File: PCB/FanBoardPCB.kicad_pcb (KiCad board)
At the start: 2 copper layers, 40 x 37.9 mm, 29 parts, among them J1 Conn_01x02_Pin, J2 Conn_01x02_Pin, J3 Conn_01x02_Pin, J4 Conn_01x02_Pin, J5 FanBrdConn, Q1 IRLML0030, Q2 IRLML0030, Q3 IRLML0030, Q4 IRLML0030

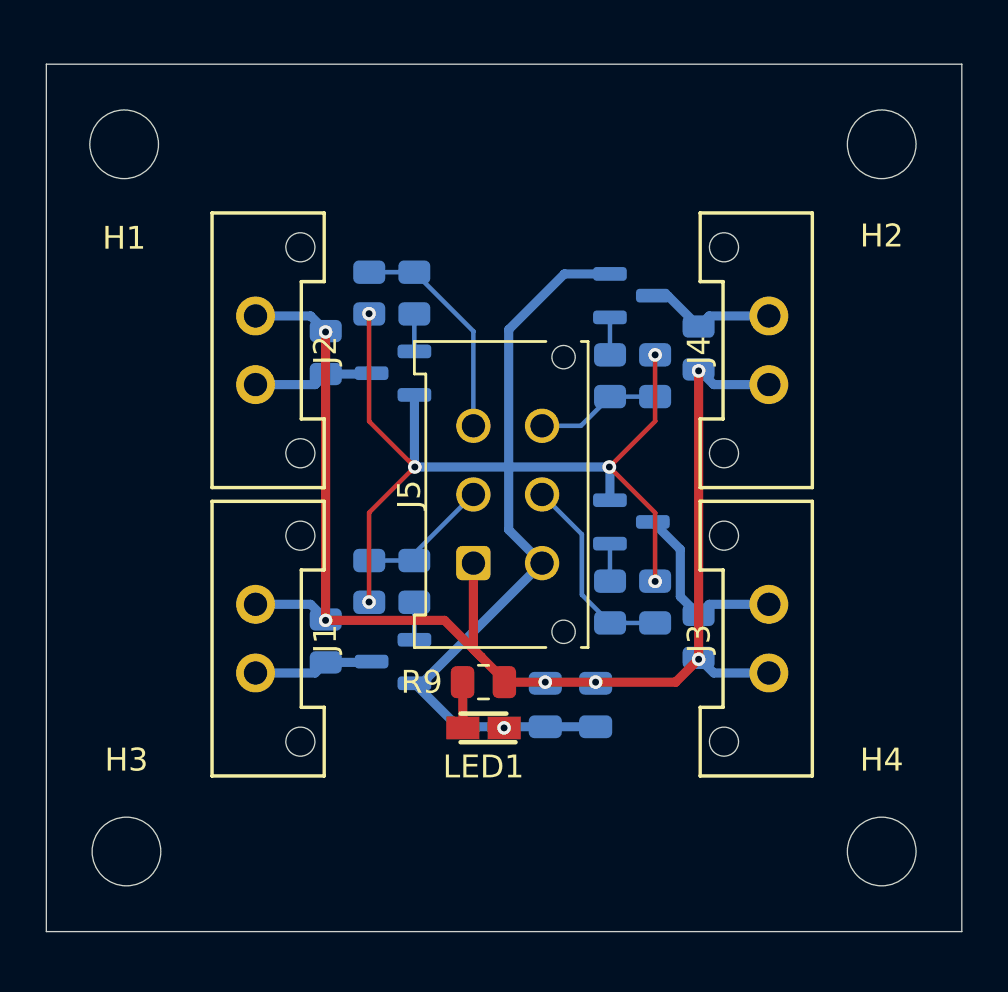
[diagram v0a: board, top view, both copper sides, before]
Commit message: fixed
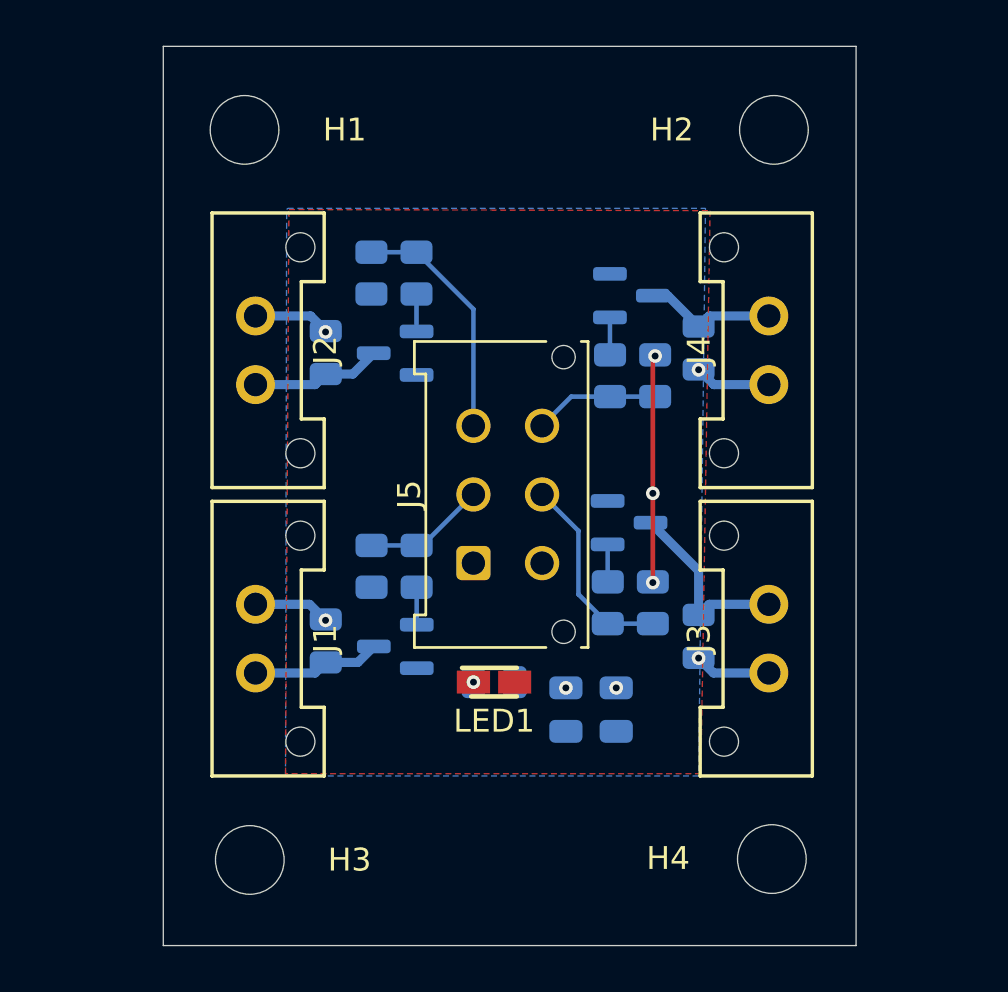
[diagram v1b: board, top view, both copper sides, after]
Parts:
- R9: moved to B.Cu
- moved H3 5.40 mm to (76.4, 130.6)
- moved H1 5.30 mm to (76.2, 98.7)
- moved H4 4.81 mm to (99.2, 130.5)
- moved H2 4.75 mm to (99.3, 98.7)
- moved LED1 2.05 mm to (87.1, 122.8), turned to 0 degrees
- moved C1 0.92 mm to (92.4, 124.0)
- moved C2 0.92 mm to (90.2, 124.0)
- moved Q2 0.88 mm to (82.7, 108.4)
- moved R3 0.88 mm to (81.7, 104.9)
- moved R4 0.88 mm to (83.7, 104.9)
- moved Q1 0.67 mm to (82.7, 121.2)
- moved R2 0.67 mm to (83.7, 117.7)
- moved R1 0.67 mm to (81.7, 117.7)
- moved R9 0.46 mm to (87.1, 122.8), turned to 0 degrees
- moved Q3 0.11 mm to (93.0, 115.8)
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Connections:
- LED1 pad 1: GNDPWR -> Net-(LED1-K)
- LED1 pad 2: Net-(LED1-A) -> +12V
- R9 pad 1: +12V -> Net-(LED1-K)
- R9 pad 2: Net-(LED1-A) -> GNDPWR
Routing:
- net GNDPWR: track 71.7 -> 9.94 mm, vias 7 -> 3
- net +12V: track 60.8 -> 13.4 mm
- net Net-(LED1-A): track 2.01 -> 0.00 mm
- net FAN2: track 9.75 -> 10.6 mm
- net FAN1: track 5.93 -> 5.37 mm
- net Net-(LED1-K): vias 0 -> 1
- added copper zone on F.Cu, net +12V
- added copper zone on B.Cu, net GNDPWR
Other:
- board size 40 x 37.9 mm -> 30.3 x 39.3 mm
